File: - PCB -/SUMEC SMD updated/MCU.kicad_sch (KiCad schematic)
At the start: 22 parts, among them J5 TYPE-C-31-M-12, SW2 SW_Push, SW3 SW_Push, U2 ESP32-S3-WROOM-1, U3 USBLC6-2SC6

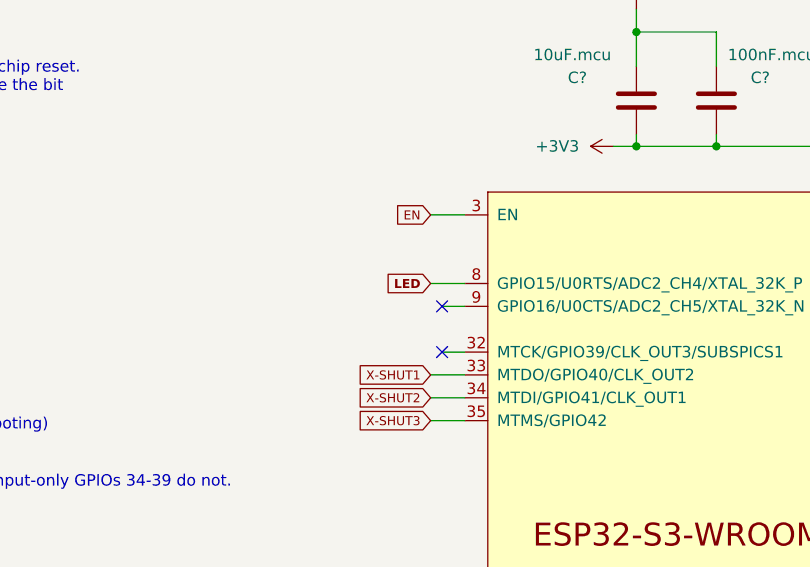
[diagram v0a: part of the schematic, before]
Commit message: cleanup sumec enchanced
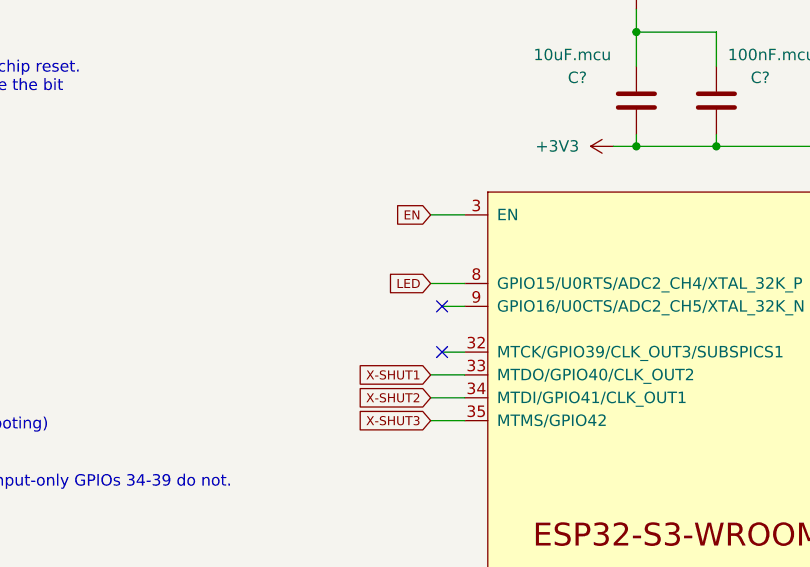
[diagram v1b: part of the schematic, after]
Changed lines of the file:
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@@
   )
   (global_label "LED" (shape input) (at 187.96 161.29 180) (fields_autoplaced)
-    (effects (font (size 1 1) bold (color 0 0 0 1)) (justify right))
-    (property "Intersheetrefs" "${INTERSHEET_REFS}" (at 182.6204 161.29 0)
+    (effects (font (size 1 1) (color 0 0 0 1)) (justify right))
+    (property "Intersheetrefs" "${INTERSHEET_REFS}" (at 182.9578 161.29 0)
       (effects (font (size 1.27 1.27)) (justify right) hide)
     )
